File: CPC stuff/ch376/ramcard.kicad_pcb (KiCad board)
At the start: 2 copper layers, 69.1 x 40.4 mm, 31 parts, among them IC1 74LS20, IC2 74LS02, IC3 74LS138, IC4 CH376, P1 CONN_25X2, P2 USB_A, P3 USB_B, U1 LD1117S33CTR, U2 CONN_SD, U3 TL16C550C, U4 FT230X, U5 74LS38

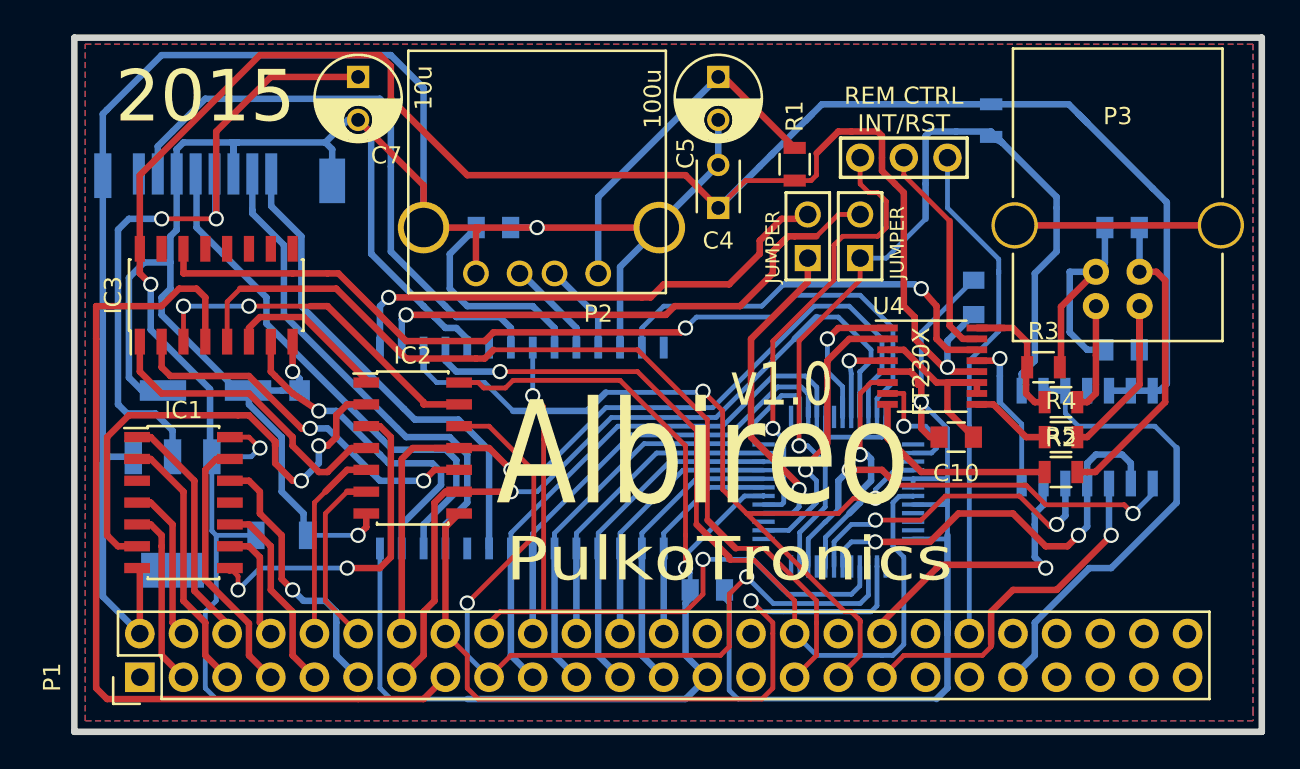
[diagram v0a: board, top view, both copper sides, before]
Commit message: A lot of tweaking and small fixes.
git-svn-id: svn://pulkomandy.tk/avrstuff@119 c6672c3c-f6b6-47f9-9001-1fd6b12fecbe
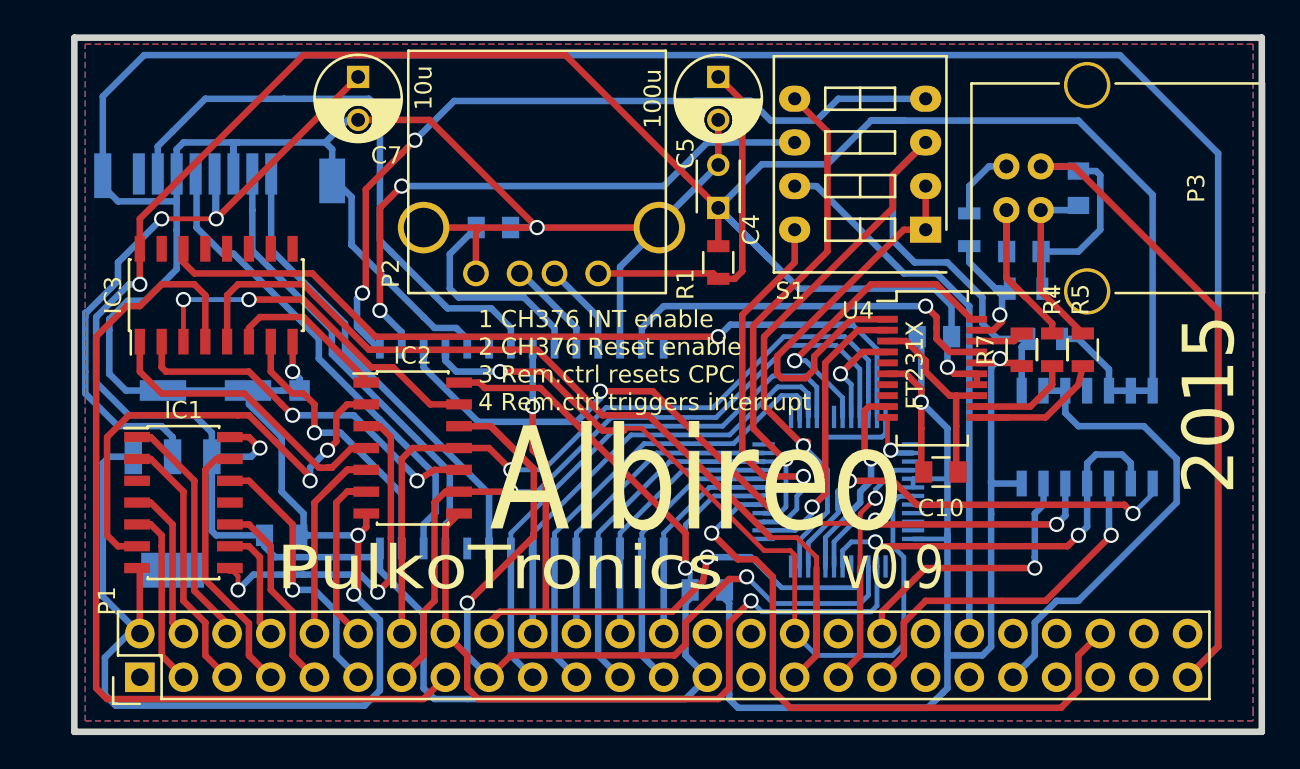
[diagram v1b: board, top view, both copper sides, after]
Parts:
- removed JP1: JUMPER3, opendous:SIL-3-Blank
- removed JP2, JP3: JUMPER, opendous:SIL-2_Opendous
- added R7: 4k7, Resistors_SMD:R_0805, F.Cu at (72.9, 48.3)
- added S1: SW_DIP_x4, Buttons_Switches_ThroughHole:SW_DIP_x4_Slide, F.Cu at (67.3, 41.3)
- C3: footprint Capacitors_SMD:C_1206 -> Capacitors_SMD:C_0805
- R2, R3: moved to B.Cu
- U4: value FT230X -> FT231X; footprint Housings_SSOP:SSOP-16_3.9x4.9mm_Pitch0.635mm -> ch376:SSOP-24_3.9x8.7mm_Pitch0.635mm
- moved R6 13.1 mm to (74.3, 47.6), turned to 180 degrees
- moved R2 11.4 mm to (69.8, 41.3), turned to 270 degrees
- moved P3 9.65 mm to (72.0, 37.6), turned to 0 degrees
- moved C9 8.08 mm to (73.0, 42.5), turned to 0 degrees
- moved R1 7.24 mm to (55.2, 43.2), turned to 90 degrees
- moved R5 7.22 mm to (76.5, 48.3), turned to 90 degrees
- moved R4 5.11 mm to (74.7, 48.3), turned to 90 degrees
- moved R3 4.68 mm to (73.2, 44.7)
- moved C8 3.42 mm to (76.2, 38.9), turned to 90 degrees
- moved C1 3.23 mm to (67.8, 47.5), turned to 180 degrees
- moved C10 2.22 mm to (68.2, 55.4)
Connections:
- IC4 pad 1: Net-(IC4-Pad1) -> /INT
- IC4 pad 2: Net-(IC4-Pad2) -> /RSTI
- P1 pad 46: (no net) -> /CURSOR
- U3 pad 39: (no net) -> //DSR
- U3 pad 41: //RI -> /CURSOR
- U4 pad 1: /RX -> /GPO2
- U4 pad 10: Net-(C10-Pad1) -> /24MHz
- U4 pad 11: Net-(C10-Pad1) -> Net-(R5-Pad1)
- U4 pad 12: VCC -> Net-(R4-Pad1)
- U4 pad 13: GND -> Net-(C10-Pad1)
- U4 pad 14: /12MHz -> VCC
- U4 pad 15: /GPO2 -> VCC
- U4 pad 16: /VBUS_Sense -> GND
- U4 pad 5: GND -> (no net)
- U4 pad 6: //RTS -> GND
- U4 pad 7: /24MHz -> (no net)
- U4 pad 8: Net-(R5-Pad1) -> (no net)
- U4 pad 9: Net-(R4-Pad1) -> //RTS
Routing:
- net GND: track 314.1 -> 437.4 mm, vias 5 -> 6
- net /INT: track 0.00 -> 49.1 mm, vias 0 -> 2
- net /CURSOR: track 0.00 -> 37.4 mm, vias 0 -> 1
- net /RSTI: track 0.00 -> 35.2 mm, vias 0 -> 2
- net VCC: track 277.8 -> 244.7 mm
- net Net-(IC4-Pad2): track 32.5 -> 0.00 mm, vias 1 -> 0
- net Net-(IC4-Pad1): track 30.0 -> 0.00 mm, vias 1 -> 0
- net //RI: track 26.9 -> 0.00 mm, vias 1 -> 0
- net //DSR: track 0.00 -> 23.1 mm, vias 0 -> 1
- net Net-(P3-Pad5): track 12.0 -> 0.00 mm
- net +3V3: track 51.6 -> 40.1 mm
- net /A1: track 48.4 -> 59.8 mm
- net /GPO2: track 12.8 -> 23.6 mm
- net /A8: track 16.8 -> 27.1 mm
- net //DCD: track 19.7 -> 28.6 mm
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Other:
- board text added: "1 CH376 INT enable 2 CH376 Reset enable 3 Rem.ctrl resets CPC 4 Rem.ctrl triggers interrupt"
- board text added: "uSD"
- board text added: "v0.9"
- board text removed: "REM CTRL INT/RST"
- board text removed: "v1.0"
